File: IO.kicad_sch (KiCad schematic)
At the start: 2 parts, among them J1 USB-C-(USB4056-03-A_REVA2)

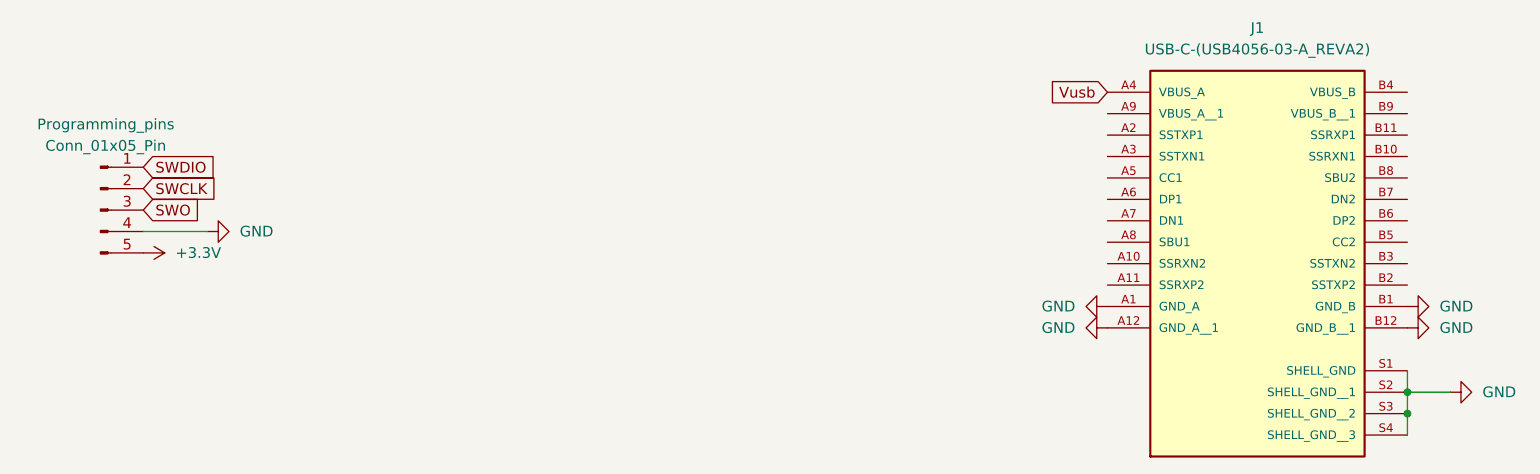
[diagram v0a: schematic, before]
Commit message: Connexion partielle du connecteur usb
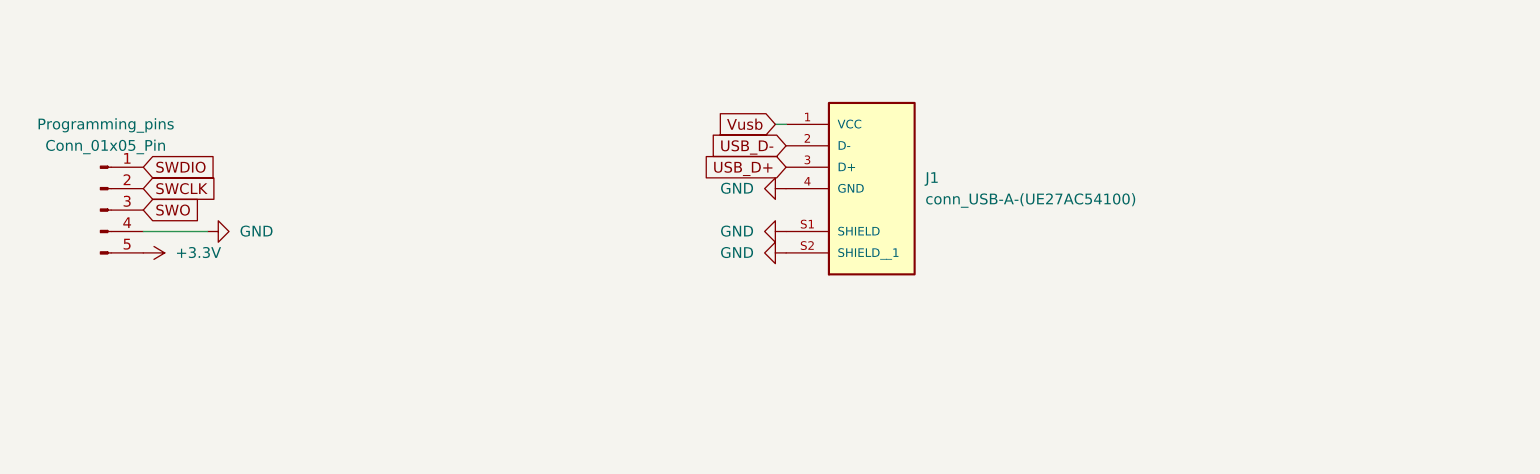
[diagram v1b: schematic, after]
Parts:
- removed J1: USB-C-(USB4056-03-A_REVA2), USB4056-03-A_REVA2:GCT_USB4056-03-A_REVA2, symbol GAUL-Symboles:USB-C-(USB4056-03-A_REVA2)
- added J1: conn_USB-A-(UE27AC54100), UE27AC54100:AMPHENOL_UE27AC54100, symbol GAUL-Symboles:conn_USB-A-(UE27AC54100)
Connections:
- net GND: now also J1.4 (GND), J1.S1 (SHIELD), J1.S2 (SHIELD__1)
- net Vusb: now also J1.1 (VCC)
- new net USB_D+: J1.3 (D+)
- new net USB_D-: J1.2 (D-)
